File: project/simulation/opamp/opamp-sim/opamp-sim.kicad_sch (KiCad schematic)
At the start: 10 parts, among them U1 OPAMP, U2 OPAMP

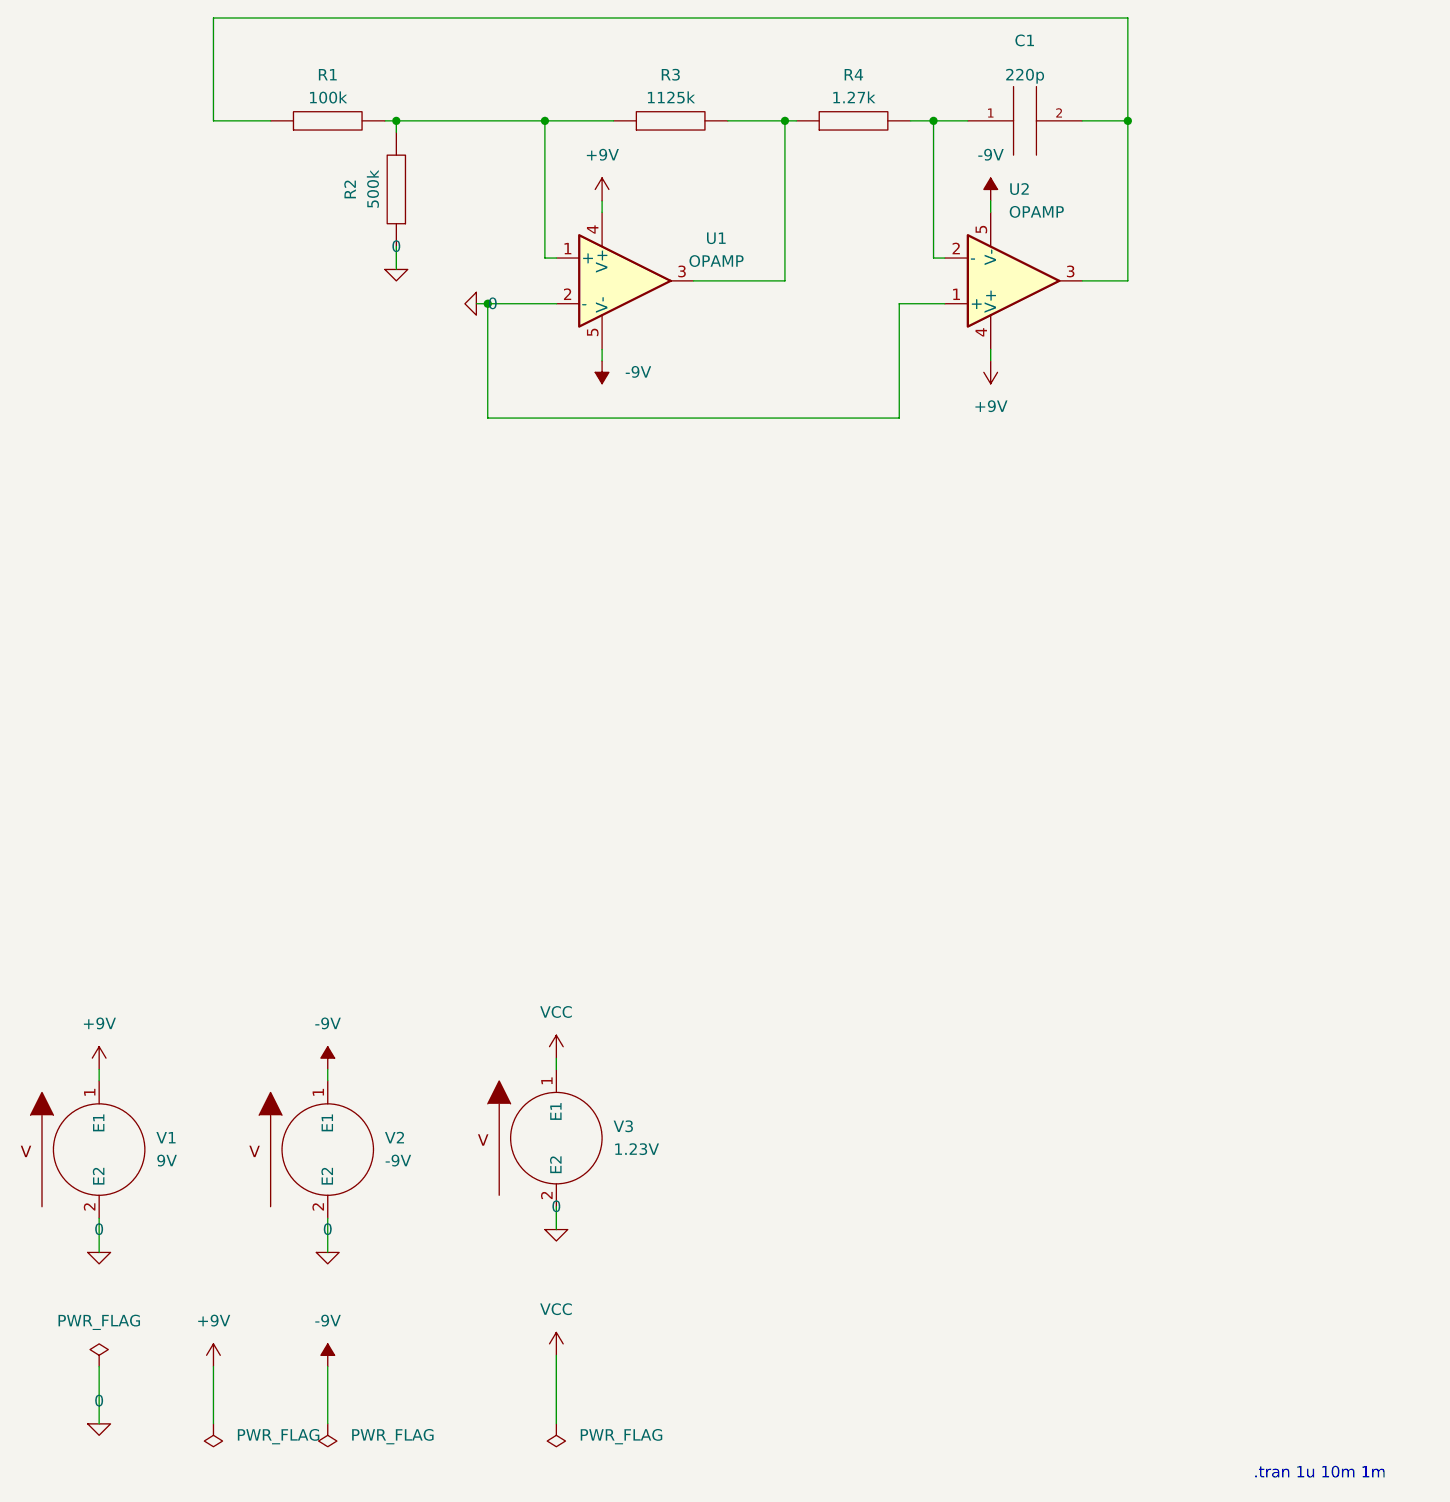
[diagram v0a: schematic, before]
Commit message: rapor hazırladım
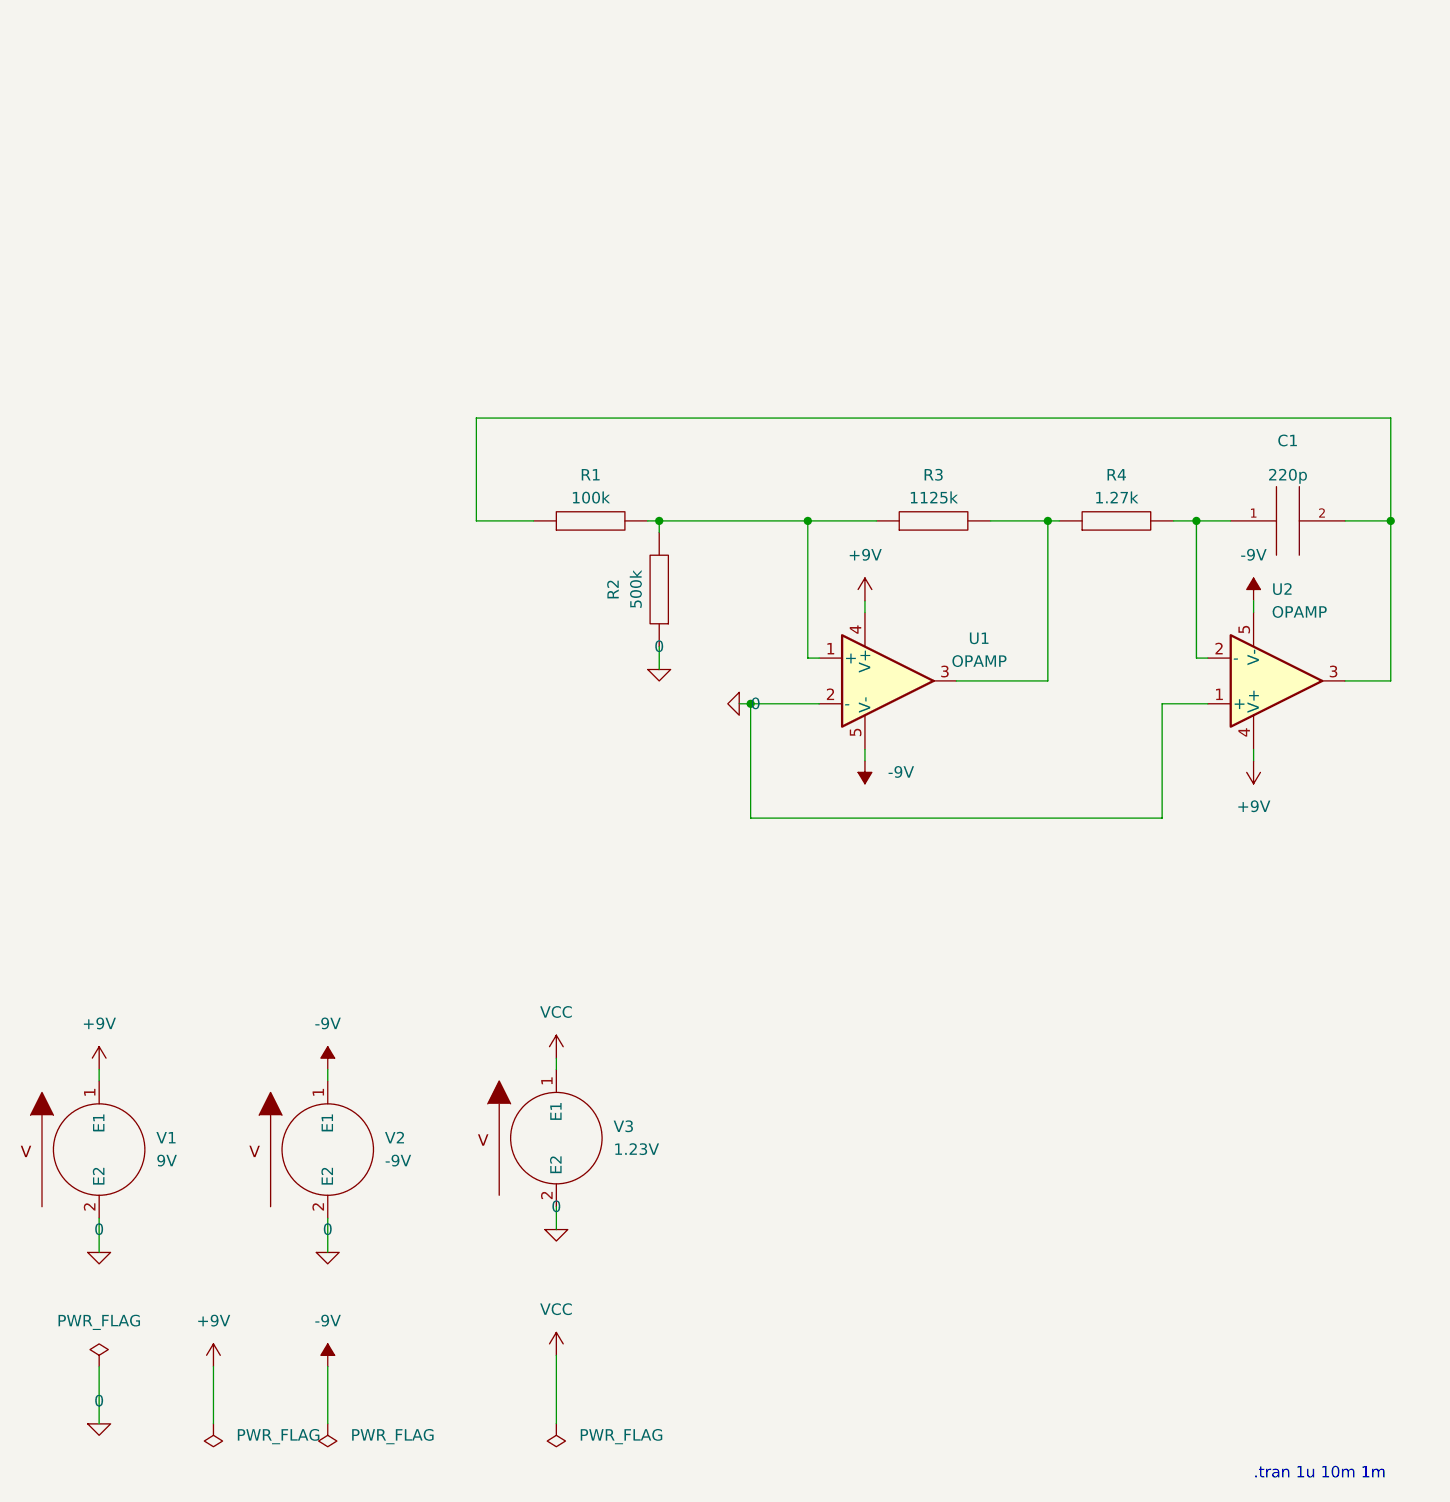
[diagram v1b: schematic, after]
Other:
- moved on the sheet: C1, R1, R2, R3, R4, U1, U2
